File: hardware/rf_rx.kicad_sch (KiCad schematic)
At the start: 29 parts, among them J5 SMA_Conn, J6 Conn_Signal, J7 Conn_Amp1, J8 Conn_Amp2, J9 Conn_TriggerOut, Q1 BC847C,215, U6 MAX4003, U7 BA4580RFVM-TR, U8 LM311

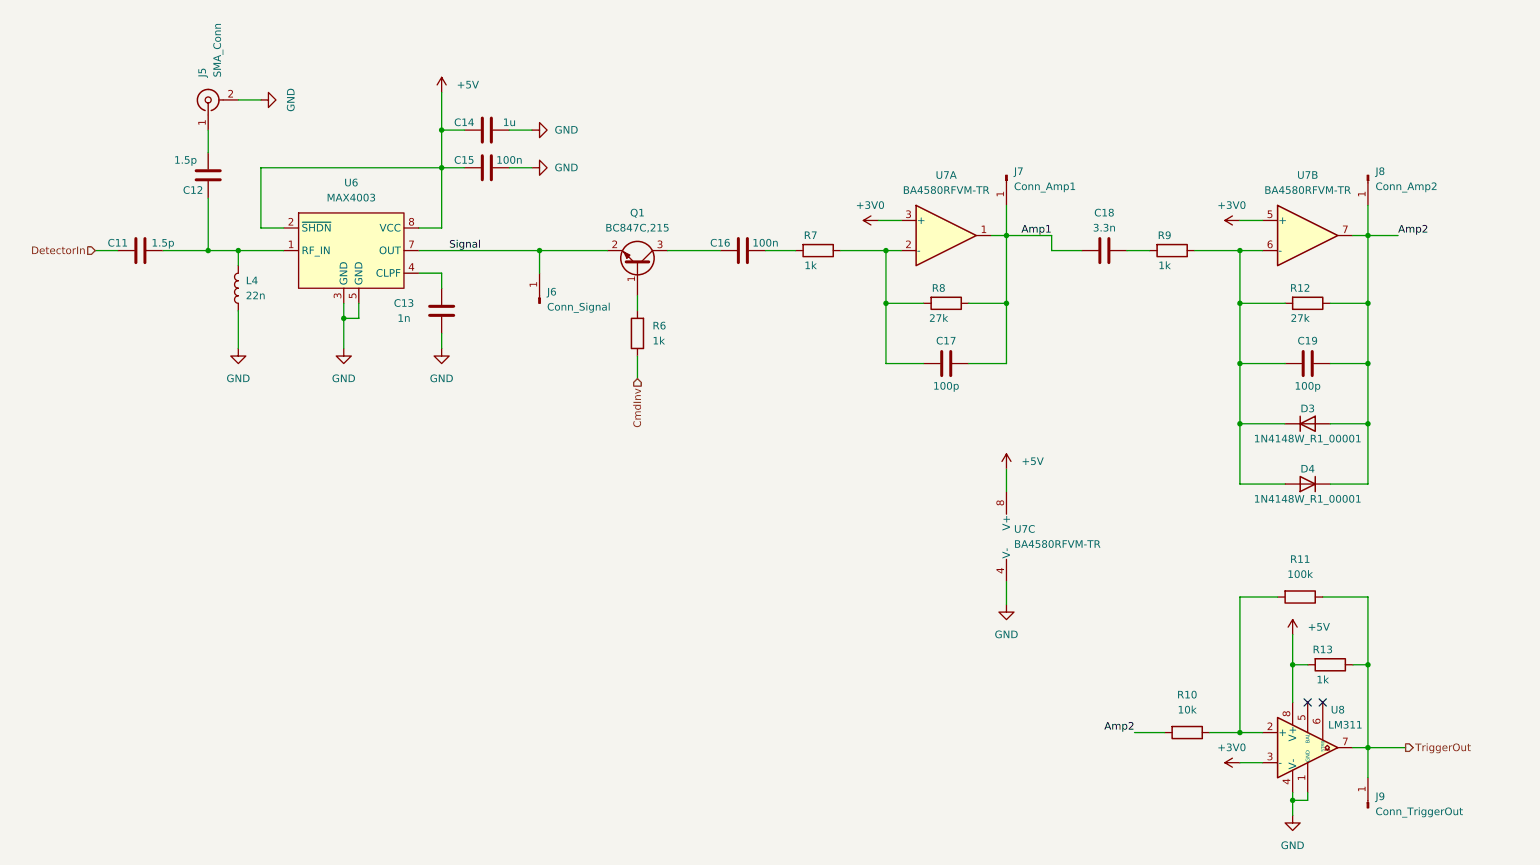
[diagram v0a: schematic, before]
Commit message: Updated schematic, PCB and fabrication files
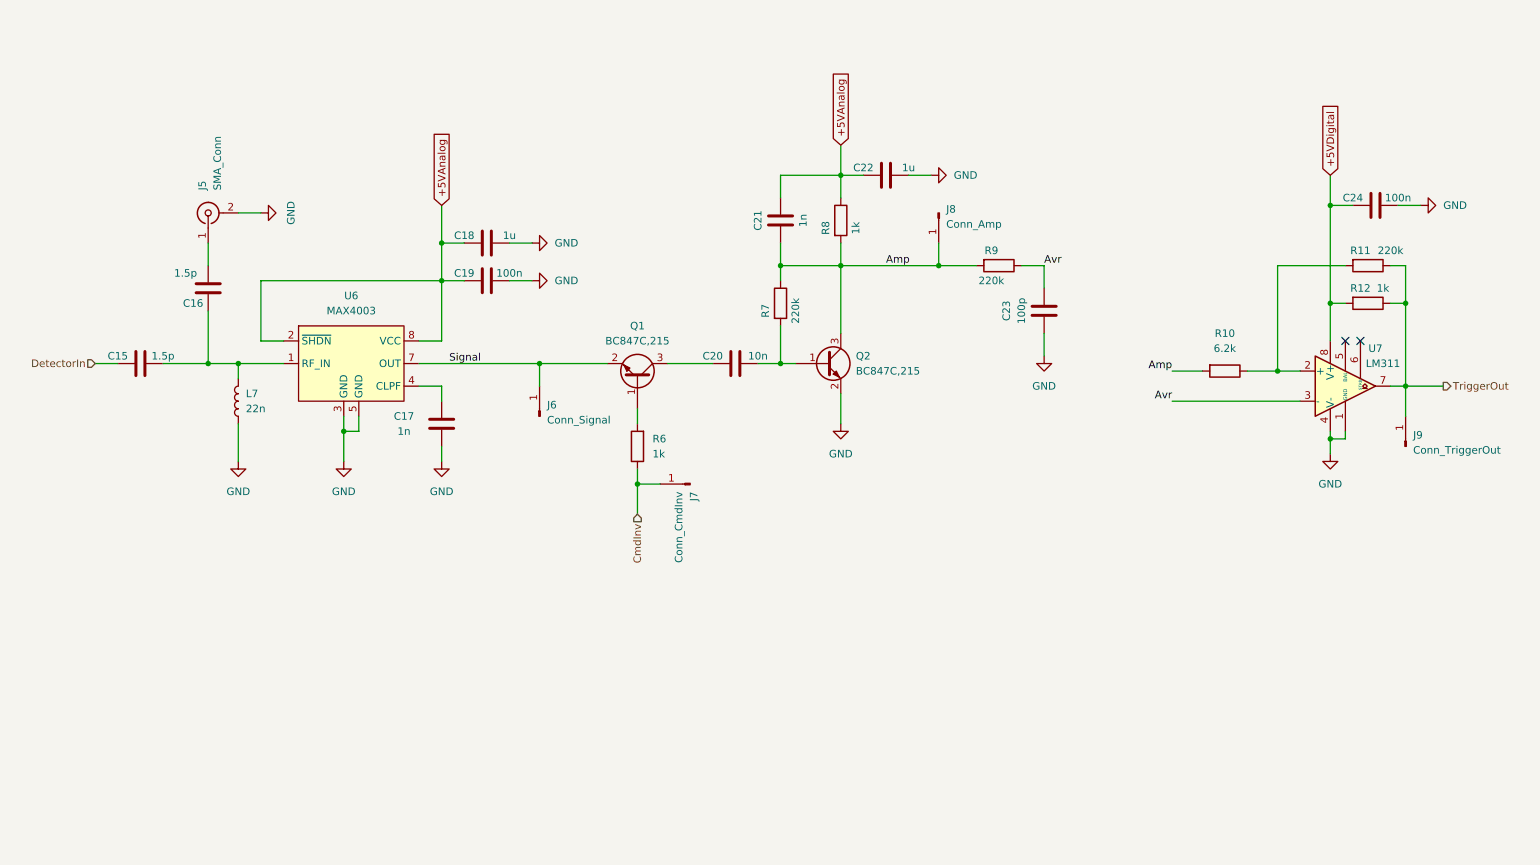
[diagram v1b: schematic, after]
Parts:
- removed C19: 100p, Capacitor_SMD:C_0603_1608Metric, symbol Device:C
- removed D3, D4: 1N4148W_R1_00001, Diode_SMD:D_SOD-123, symbol Diode:1N4148W
- removed R12: 27k, Resistor_SMD:R_0603_1608Metric, symbol Device:R
- removed U7: BA4580RFVM-TR, Package_SO:MSOP-8_3x3mm_P0.65mm, symbol Amplifier_Operational:LM358
- added C22: 1u, Capacitor_SMD:C_0603_1608Metric, symbol Device:C
- added C24: 100n, Capacitor_SMD:C_0603_1608Metric, symbol Device:C
- added Q2: BC847C,215, Package_TO_SOT_SMD:SOT-23, symbol Transistor_BJT:BC847
- C20: renamed from C16; value 100n -> 10n
- C21: renamed from C17; value 100p -> 1n
- C23: renamed from C18; value 3.3n -> 100p
- J7: renamed from J8; value Conn_Amp2 -> Conn_CmdInv
- J8: renamed from J7; value Conn_Amp1 -> Conn_Amp
- R10: value 10k -> 6.2k
- R11: value 100k -> 220k
- R7, R9: value 1k -> 220k
- R8: value 27k -> 1k
- renumbered C11 to C15, C12 to C16, C13 to C17, C14 to C18, C15 to C19, L4 to L7, R13 to R12, U8 to U7
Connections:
- net +3V0 is gone; now on net Avr: U7.3 (-)
- net CmdInv: now also J7.1 (Pin_1)
- net GND: now also C23.2, C22.1, C24.1, Q2.2 (E)
- net Amp: now reaches C21.2, R7.1, R8.2
- net Amp: now also J8.1 (Pin_1), R10.2, R9.2, Q2.3 (C)
- net Avr: now reaches R9.1
- net Avr: now also C23.1
- net at C20.1, R7.2: now also Q2.1 (B)
- net +5V renamed +5VAnalog
- net +5VAnalog: now also C21.1, R8.1, C22.2; no longer R12.2, U7.8 (V+)
- removed net Amp1: C21.1, C23.2, J8.1 (Pin_1), R8.1
- removed net Amp2: J7.1 (Pin_1), R10.2
- new net +5VDigital: C24.2, R12.2, U7.8 (V+)
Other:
- moved on the sheet: C15, C16, C17, C18, C19, C20, C21, C23, J5, J6, J7, J8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
